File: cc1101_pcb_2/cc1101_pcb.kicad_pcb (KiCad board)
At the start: 2 copper layers, 24 x 22 mm, 8 parts, among them J1 Conn_01x08_MountingPin, J2 Conn_01x08_MountingPin, J3 Conn_02x04_Odd_Even_Shielded

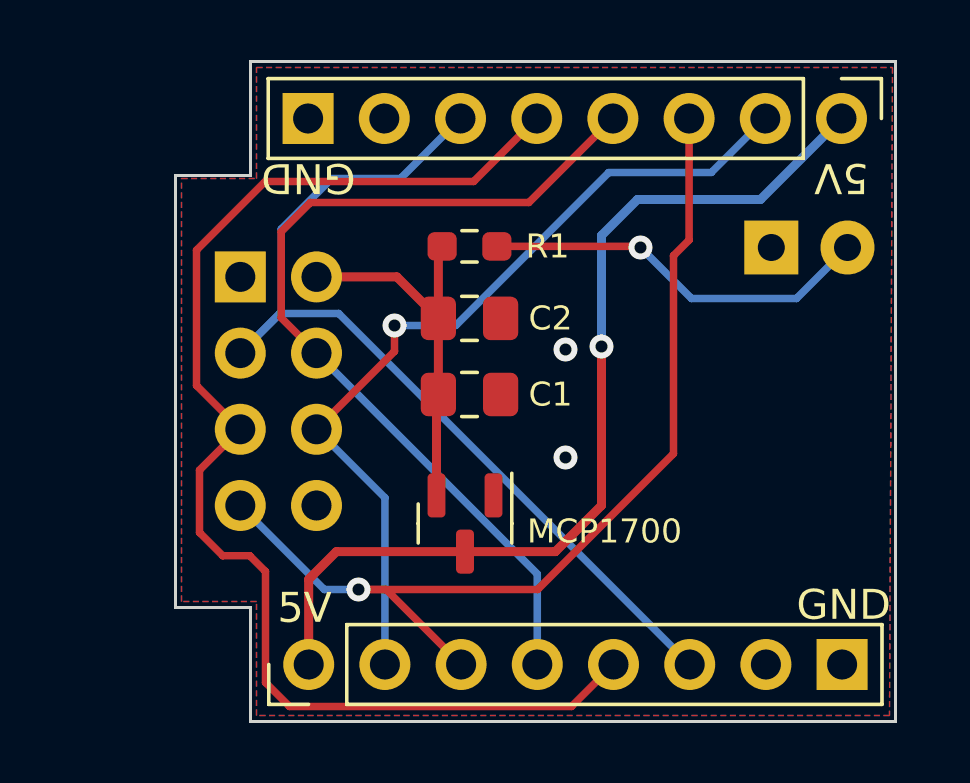
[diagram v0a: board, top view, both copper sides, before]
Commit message: Modifiche varie che non voglio controllare
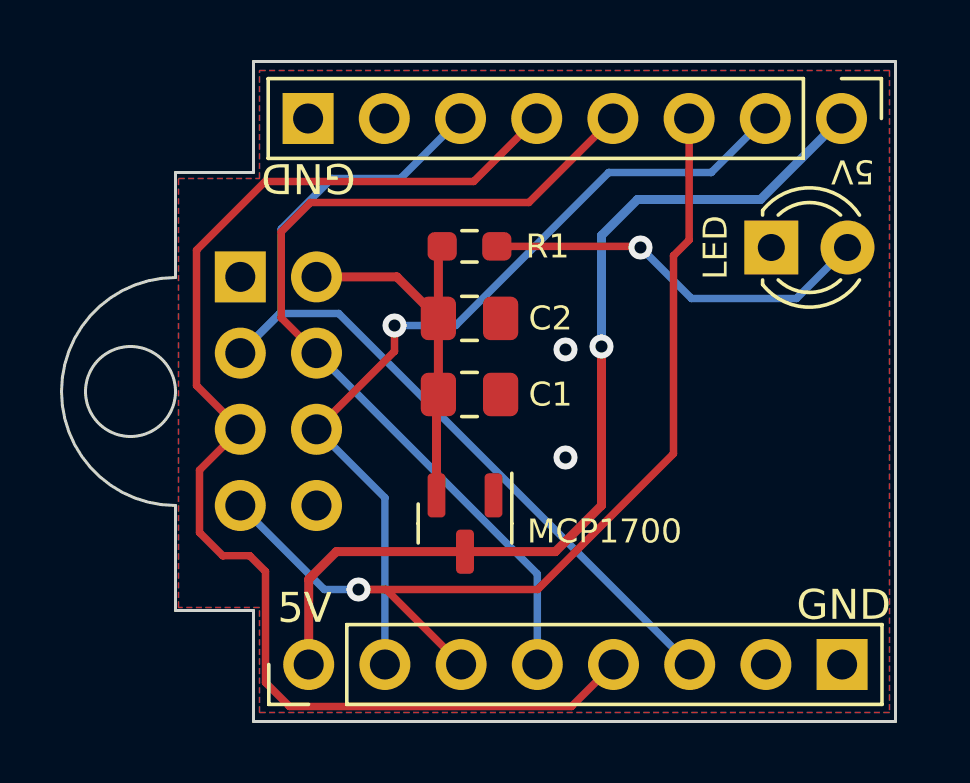
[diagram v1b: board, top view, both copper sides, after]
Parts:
- LED: moved to F.Cu
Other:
- board size 24 x 22 mm -> 27.8 x 22 mm
